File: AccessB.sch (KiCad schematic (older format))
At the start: 11 parts, among them P1 ICSP, P2 USB_OTG, P3 GPIO, P5 USB_OTG, U1 PIC18(L)F2550-I/SO, Y1 4MHz

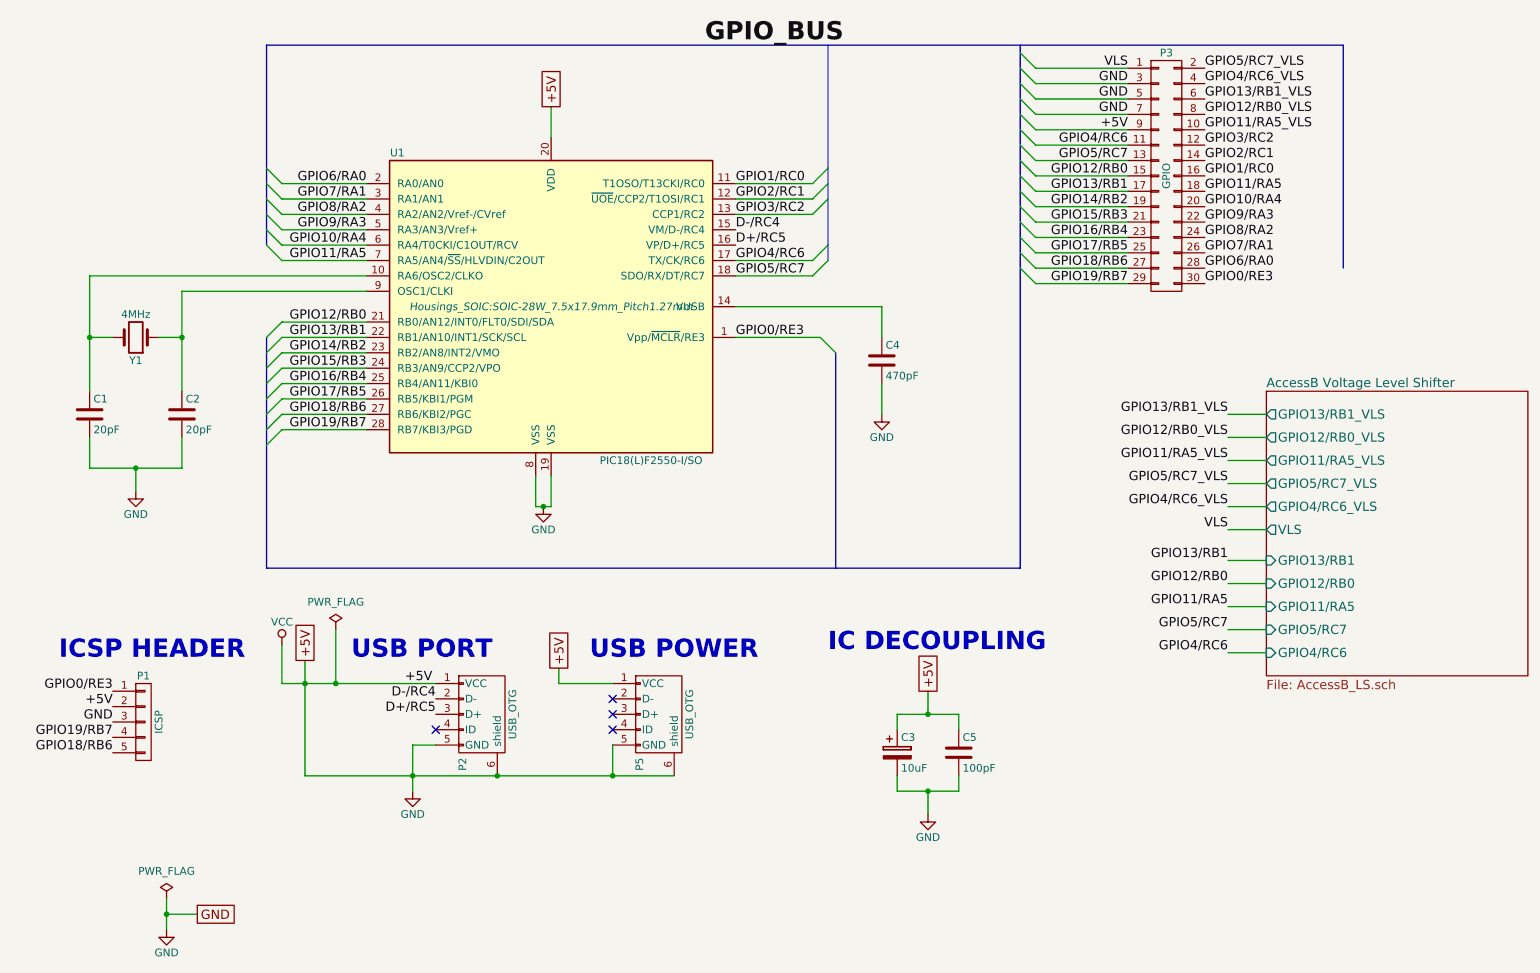
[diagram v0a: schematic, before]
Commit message: update
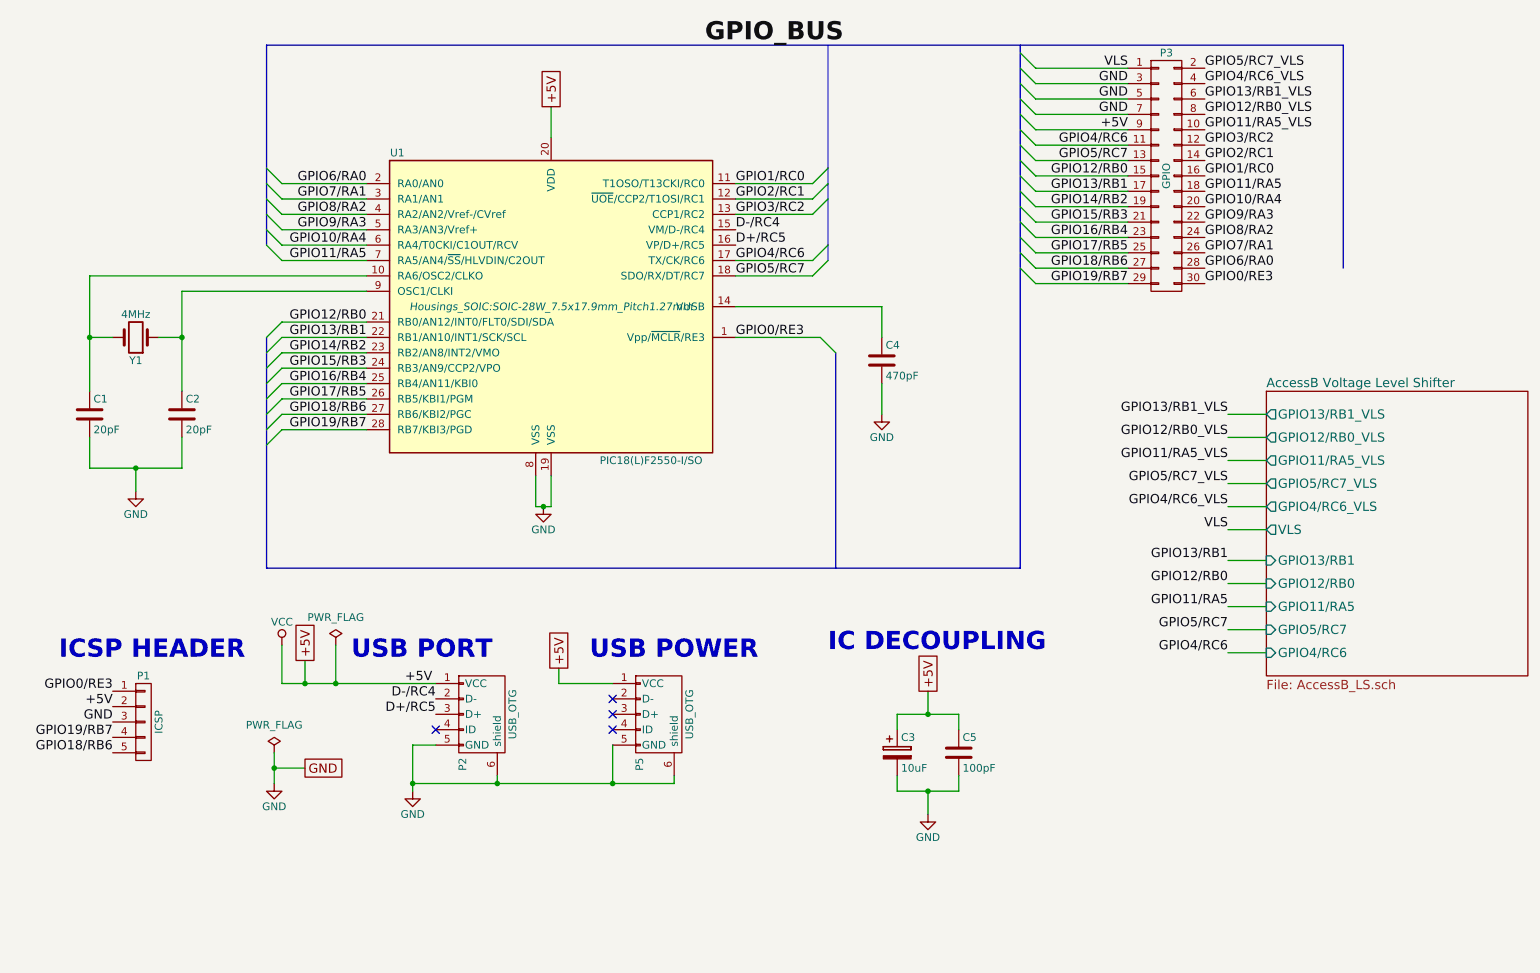
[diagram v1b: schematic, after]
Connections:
- net GND: no longer C3.1, C5.1, P1.2 (P2), P2.1 (VCC), P3.9 (P9), P5.1 (VCC), U1.20 (VDD)
- new net VCC: C3.1, C5.1, P1.2 (P2), P2.1 (VCC), P3.9 (P9), P5.1 (VCC), U1.20 (VDD)
